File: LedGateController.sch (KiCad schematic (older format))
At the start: 49 parts, among them J1 GPIO, J2 SWD, J3 LED_OUT, Q1 FS8205A, Q2 AO3400A, Q3 AO3401A, SW1 BUTTON, SW2 ON_OFF, U1 STM32F030F4Px, U2 MT3608, U3 DW01, U4 XC6206P332MR, U5 PI4ULS5V201

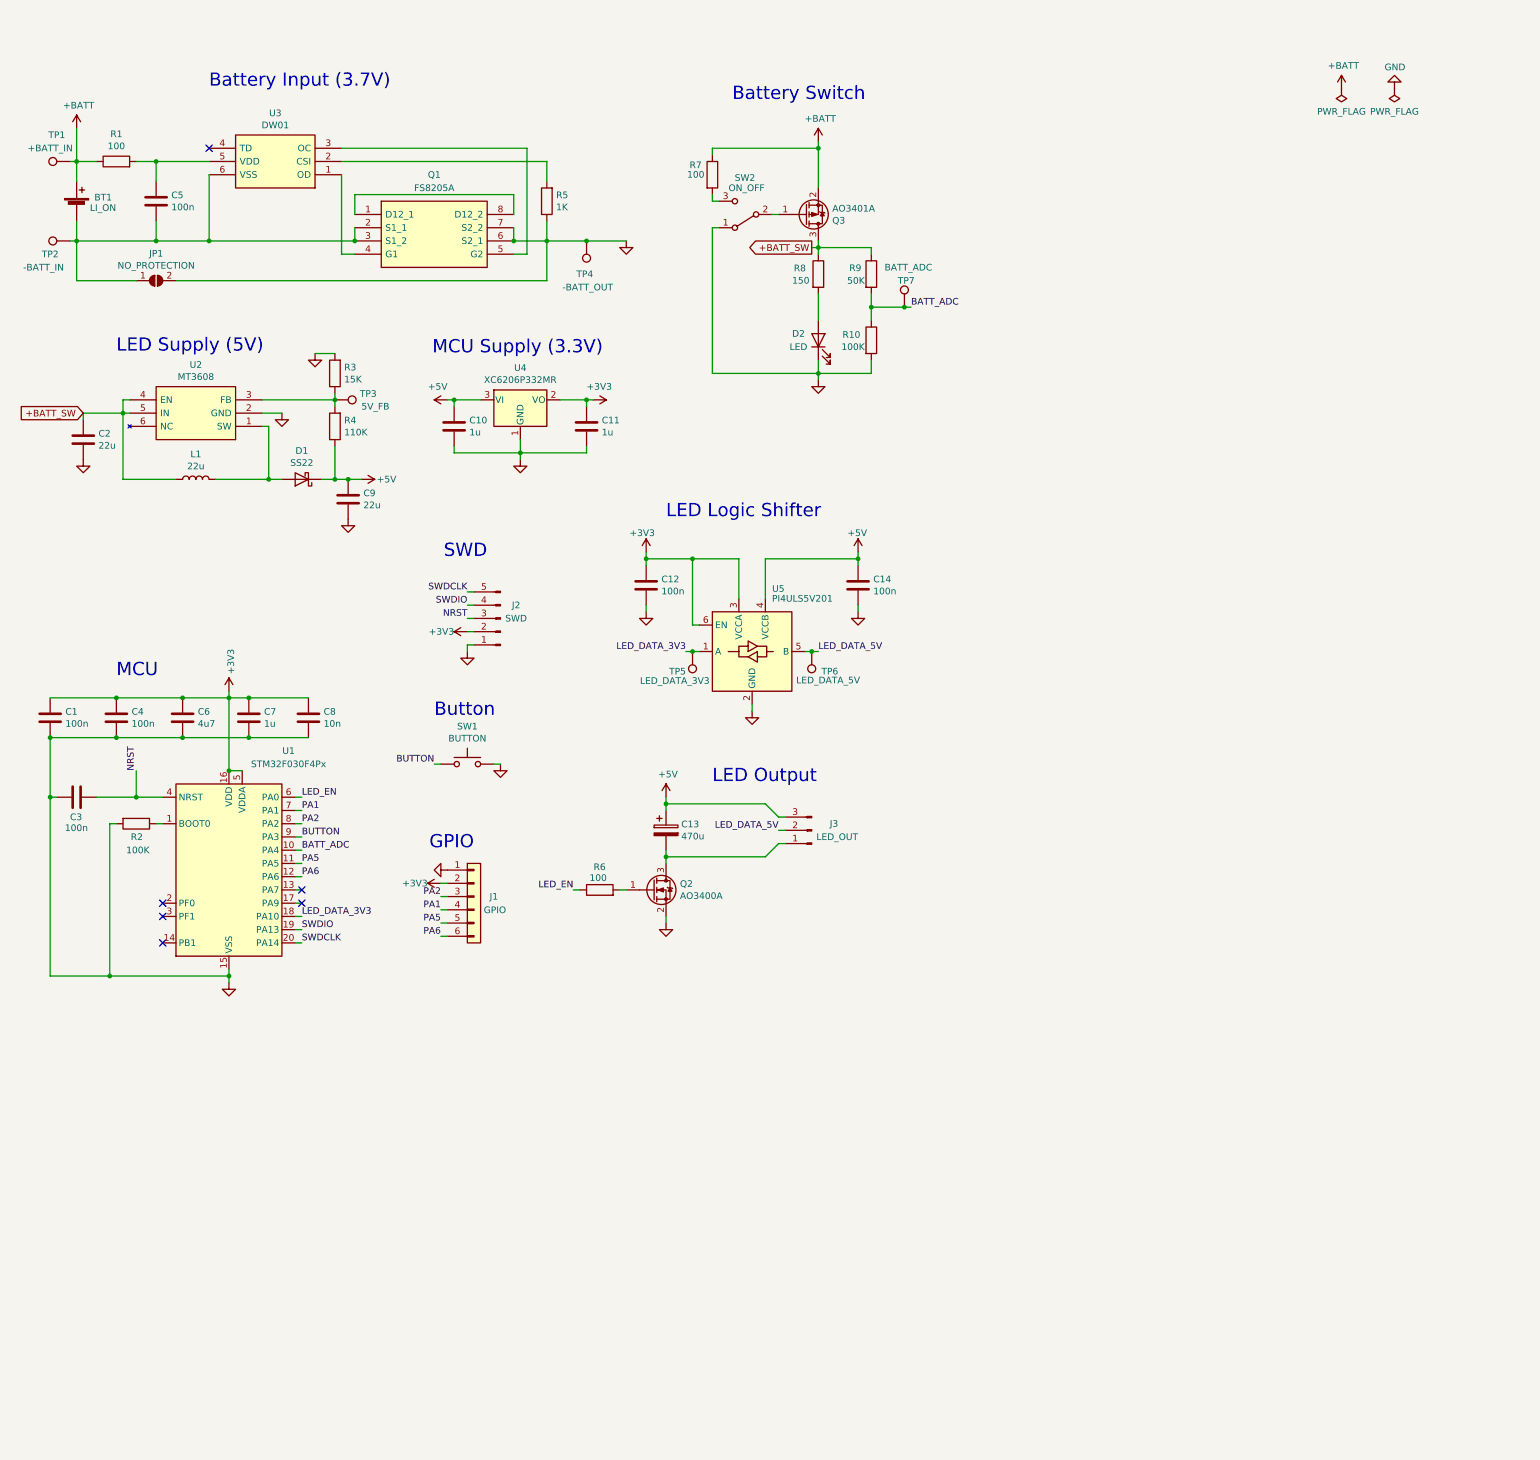
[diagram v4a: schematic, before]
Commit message: Update schematic
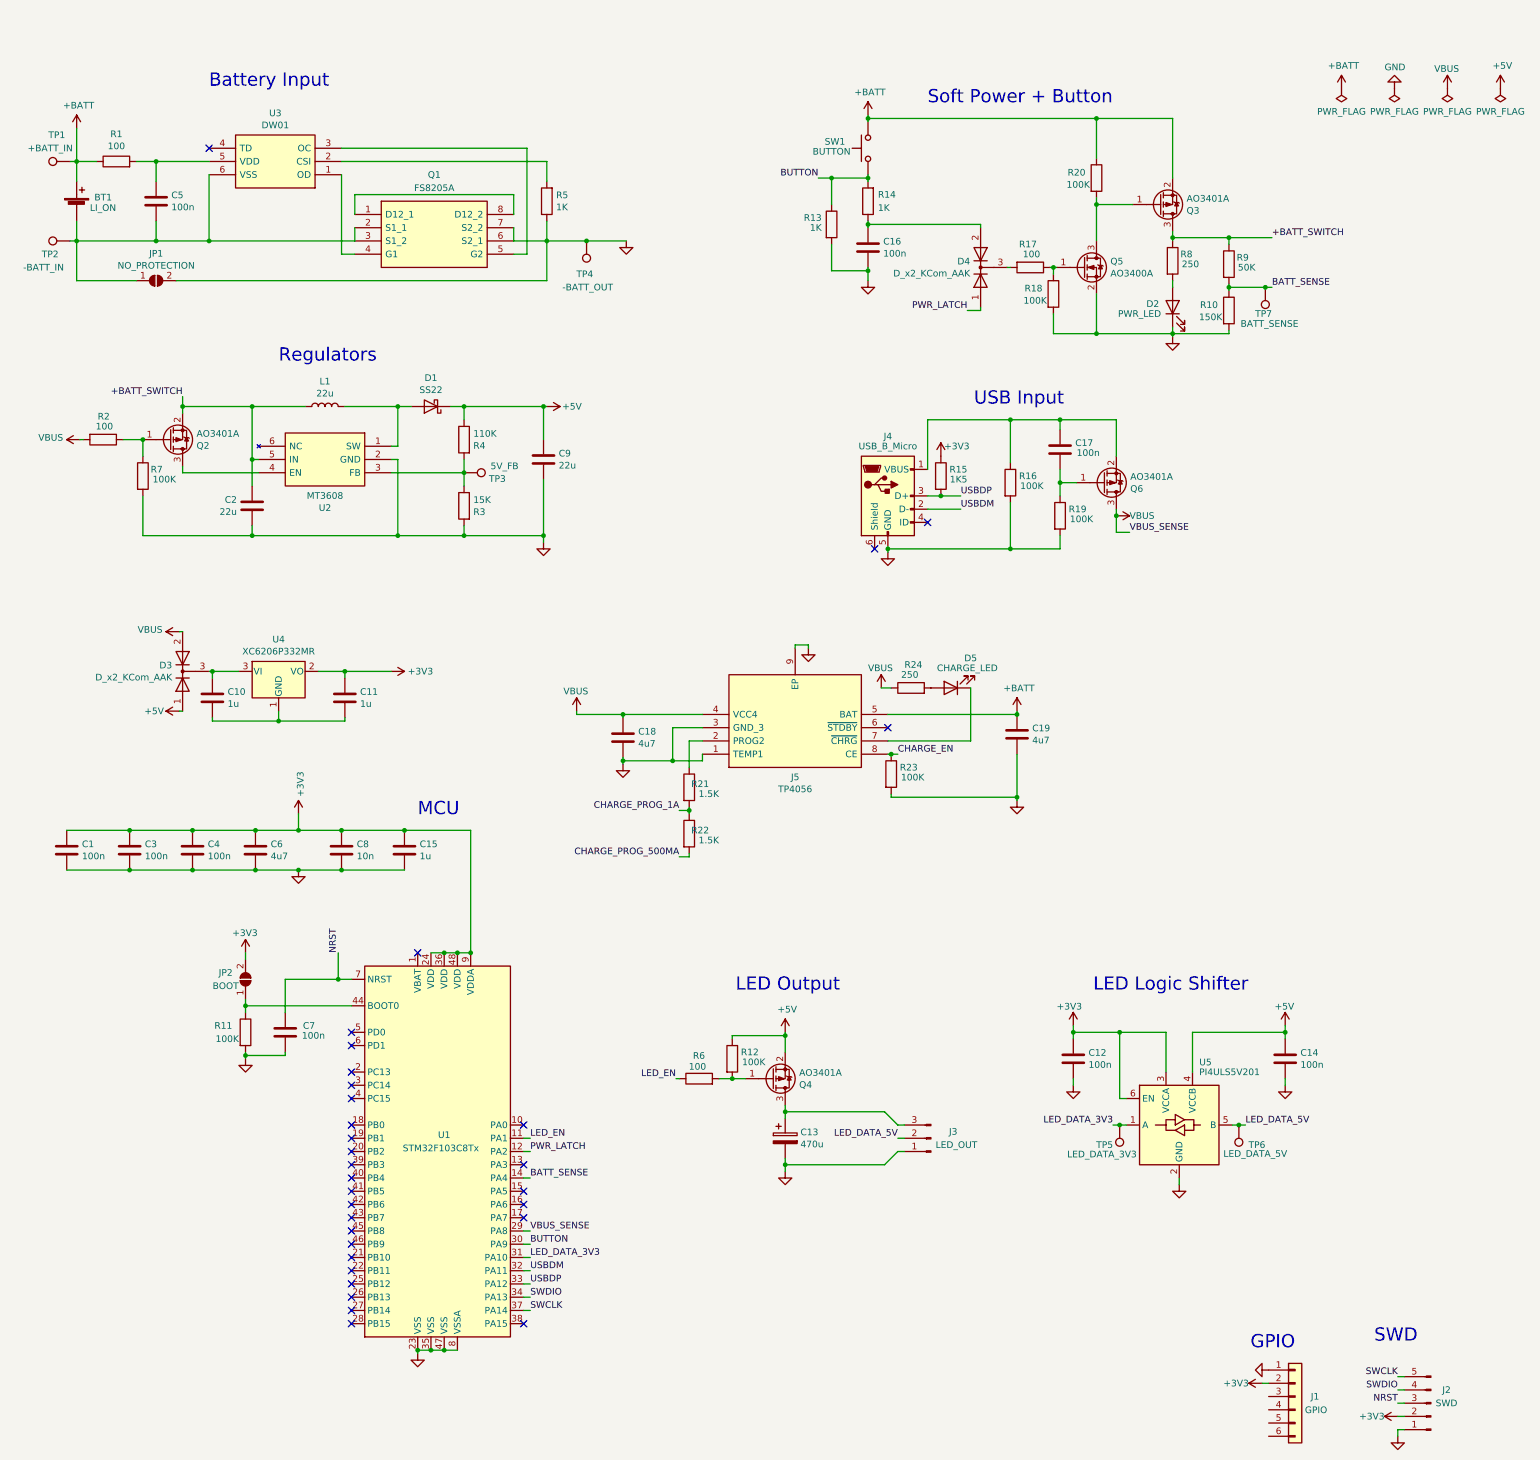
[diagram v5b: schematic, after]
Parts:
- removed Q2: AO3400A, Package_TO_SOT_SMD:SOT-23, symbol MiscParts:AO3400A
- removed SW2: ON_OFF, SamacSys_Parts:SK12D07VG4NSPA, symbol Switch:SW_SPDT
- removed U1: STM32F030F4Px, Package_SO:TSSOP-20_4.4x6.5mm_P0.65mm, symbol MCU_ST_STM32F0:STM32F030F4Px
- added C15: 1u, Capacitor_SMD:C_0805_2012Metric, symbol Device:C
- added C16, C17: 100n, Capacitor_SMD:C_0805_2012Metric, symbol Device:C
- added C18, C19: 4u7, Capacitor_SMD:C_0805_2012Metric, symbol Device:C
- added D3, D4: D_x2_KCom_AAK, Package_TO_SOT_SMD:SOT-23, symbol Device:D_x2_KCom_AAK
- added D5: CHARGE_LED, LED_SMD:LED_0805_2012Metric, symbol Device:LED
- added J4: USB_B_Micro, SamacSys_Parts:U254051T4BHJ25S2S, symbol Connector:USB_B_Micro
- added J5: TP4056, SamacSys_Parts:SOIC127P600X175-9N, symbol SamacSys_Parts:TP4056
- added JP2: BOOT, Jumper:SolderJumper-2_P1.3mm_Open_Pad1.0x1.5mm, symbol Jumper:SolderJumper_2_Open
- added Q2, Q4, Q6: AO3401A, Package_TO_SOT_SMD:SOT-23, symbol Transistor_FET:AO3401A
- added Q5: AO3400A, Package_TO_SOT_SMD:SOT-23, symbol MiscParts:AO3400A
- added R11, R12, R16, R18, R19, R20, R23: 100K, Resistor_SMD:R_0805_2012Metric, symbol Device:R
- added R13, R14: 1K, Resistor_SMD:R_0805_2012Metric, symbol Device:R
- added R15: 1K5, Resistor_SMD:R_0805_2012Metric, symbol Device:R
- added R17: 100, Resistor_SMD:R_0805_2012Metric, symbol Device:R
- added R21, R22: 1.5K, Resistor_SMD:R_0805_2012Metric, symbol Device:R
- added R24: 250, Resistor_SMD:R_0805_2012Metric, symbol Device:R
- added U1: STM32F103C8Tx, Package_QFP:LQFP-48_7x7mm_P0.5mm, symbol MCU_ST_STM32F1:STM32F103C8Tx
- C1, C10, C11, C12, C14, C2, C3, C4, C5, C6, C8, C9: footprint Capacitor_SMD:C_0805_2012Metric_Pad1.15x1.40mm_HandSolder -> Capacitor_SMD:C_0805_2012Metric
- C7: value 1u -> 100n; footprint Capacitor_SMD:C_0805_2012Metric_Pad1.15x1.40mm_HandSolder -> Capacitor_SMD:C_0805_2012Metric; LCSC Part (none) -> https://lcsc.com/product-detail/Multilayer-Ceramic-Capacito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
- D2: value LED -> PWR_LED; footprint LED_SMD:LED_0805_2012Metric_Pad1.12x1.40mm_HandSolder -> LED_SMD:LED_0805_2012Metric
- R1, R3, R4, R5, R6, R9: footprint Resistor_SMD:R_0805_2012Metric_Pad1.15x1.40mm_HandSolder -> Resistor_SMD:R_0805_2012Metric
- R10: value 100K -> 150K; footprint Resistor_SMD:R_0805_2012Metric_Pad1.15x1.40mm_HandSolder -> Resistor_SMD:R_0805_2012Metric
- R2: value 100K -> 100; footprint Resistor_SMD:R_0805_2012Metric_Pad1.15x1.40mm_HandSolder -> Resistor_SMD:R_0805_2012Metric; LCSC Part https://lcsc.com/product-detail/Chip-Resistor-Surface-Mount_Uniroyal-Elec-0805W8F1003T5E_C17407.html/?href=jlc-SMT -> https://lcsc.com/product-detail/Chip-Resistor-Surface-Mount_Uniroyal-Elec-0805W8F1502T5E_C17475.html/?href=jlc-SMT
- R7: value 100 -> 100K; footprint Resistor_SMD:R_0805_2012Metric_Pad1.15x1.40mm_HandSolder -> Resistor_SMD:R_0805_2012Metric; LCSC Part https://lcsc.com/product-detail/Chip-Resistor-Surface-Mount_Uniroyal-Elec-0805W8F1000T5E_C17408.html/?href=jlc-SMT -> https://lcsc.com/product-detail/Chip-Resistor-Surface-Mount_Uniroyal-Elec-0805W8F1502T5E_C17475.html/?href=jlc-SMT
- R8: value 150 -> 250; footprint Resistor_SMD:R_0805_2012Metric_Pad1.15x1.40mm_HandSolder -> Resistor_SMD:R_0805_2012Metric
- TP7: value BATT_ADC -> BATT_SENSE
- U2, U3, U5: footprint Package_TO_SOT_SMD:SOT-23-6_Handsoldering -> Package_TO_SOT_SMD:SOT-23-6
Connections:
- net +3V3: now also C3.1, C15.1, JP2.2 (B), R15.1, U1.24 (VDD), U1.36 (VDD), U1.48 (VDD), U1.9 (VDDA); no longer C7.1
- net +5V: now also D3.1 (A), Q4.2 (S), R12.1; no longer C10.1, C13.1, J3.3 (Pin_3), U4.3 (VI)
- net +BATT: now also SW1.2, C19.1, J5.5 (BAT), R20.1; no longer R7.1
- net BUTTON: now also R13.1, R14.2, U1.30 (PA9)
- net GND: now also C13.2, C7.1, J3.1 (Pin_1), R7.2, C15.2, C16.2, C18.2, C19.2, J4.5 (GND), J5.1 (TEMP1), J5.3 (GND_3), J5.9 (EP), Q5.2 (S), R11.2, R13.2, R16.2, R18.2, R19.2, R23.2, U1.23 (VSS), U1.35 (VSS), U1.47 (VSS), U1.8 (VSSA); no longer C10.2, C11.2, C7.2, R2.2, SW1.2, U4.1 (GND)
- net LED_DATA_3V3: now also U1.31 (PA10)
- net LED_EN: now also U1.11 (PA1)
- net NRST: now also C7.2, U1.7 (NRST); no longer C3.1
- net SWDIO: now also U1.34 (PA13)
- net at R6.2: now also Q4.1 (G), R12.2
- net at Q3.1 (G): now also Q5.3 (D), R20.2
- net at R2.1: now also R7.1, Q2.1 (G)
- net +BATT_SW renamed +BATT_SWITCH
- net +BATT_SWITCH: now also Q2.2 (S); no longer U2.4 (EN)
- net BATT_ADC renamed BATT_SENSE
- net BATT_SENSE: now also U1.14 (PA4)
- net PA1: no longer names the net of J1.4 (Pin_4)
- net PA2: no longer names the net of J1.3 (Pin_3)
- net PA5: no longer names the net of J1.5 (Pin_5)
- net PA6: no longer names the net of J1.6 (Pin_6)
- net SWDCLK renamed SWCLK
- net SWCLK: now also U1.37 (PA14)
- new net: Q2.3 (D), U2.4 (EN)
- new net: C13.1, J3.3 (Pin_3), Q4.3 (D)
- new net: C10.1, D3.3 (K), U4.3 (VI)
- new net: C10.2, C11.2, U4.1 (GND)
- new net: JP2.1 (A), R11.1, U1.44 (BOOT0)
- new net: C17.1, J4.1 (VBUS), Q6.2 (S), R16.1
- new net: C16.1, D4.2 (A), R14.1
- new net: D4.3 (K), R17.2
- new net: Q5.1 (G), R17.1, R18.1
- new net: J5.2 (PROG2), R21.1
- new net: D5.1 (K), J5.7 (~CHRG)
- new net: D5.2 (A), R24.2
- new net: C17.2, Q6.1 (G), R19.1
- new net CHARGE_EN: J5.8 (CE), R23.1
- new net CHARGE_PROG_1A: R21.2, R22.1
- new net CHARGE_PROG_500MA: R22.2
- new net PWR_LATCH: D4.1 (A), U1.12 (PA2)
- new net USBDM: J4.2 (D-), U1.32 (PA11)
- new net USBDP: J4.3 (D+), R15.2, U1.33 (PA12)
- new net VBUS: C18.1, D3.2 (A), J5.4 (VCC4), Q6.3 (D), R2.2, R24.1, U1.29 (PA8)
- no-connect marks 6 -> 32
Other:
- note added: "Battery Input"
- note added: "Regulators"
- note added: "Soft Power + Button"
- note added: "USB Input"
- note removed: "Battery Input (3.7V)"
- note removed: "Battery Switch"
- note removed: "Button"
- note removed: "LED Supply (5V)"
- note removed: "MCU Supply (3.3V)"
- moved on the sheet: C10, C11, C12, C13, C14, C2, C9, D1, D2, J1, J2, J3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
